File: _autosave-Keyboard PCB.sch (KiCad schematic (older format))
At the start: 150 parts, among them SW1 SW_Push, U1 ATmega32U4-AU, Y1 16MHz

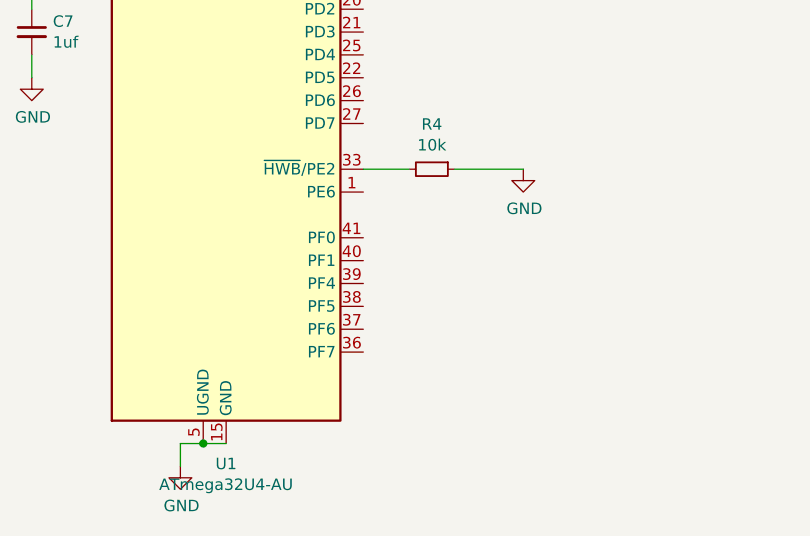
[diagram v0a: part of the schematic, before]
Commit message: column traces
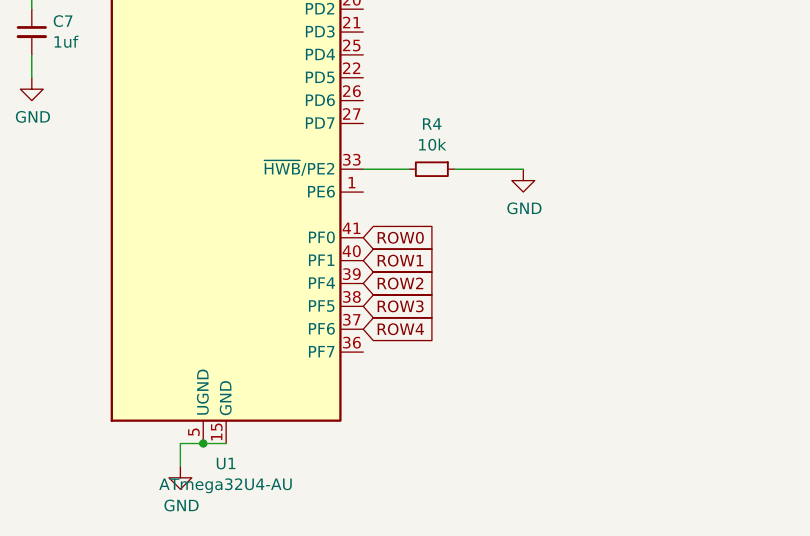
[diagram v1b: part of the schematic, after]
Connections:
- net ROW0: now also U1.41 (PF0)
- net ROW1: now also U1.40 (PF1)
- net ROW2: now also U1.39 (PF4)
- net ROW3: now also U1.38 (PF5)
- net ROW4: now also U1.37 (PF6)
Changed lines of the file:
@@
 	9450 1950 9050 1950
 Connection ~ 9050 2000
+Text GLabel 3100 6500 2    50   Input ~ 0
+ROW4
+Text GLabel 3100 6400 2    50   Input ~ 0
+ROW3
+Text GLabel 3100 6300 2    50   Input ~ 0
+ROW2
+Text GLabel 3100 6200 2    50   Input ~ 0
+ROW1
+Text GLabel 3100 6100 2    50   Input ~ 0
+ROW0
 $EndSCHEMATC
